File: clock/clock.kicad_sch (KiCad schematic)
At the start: 15 parts, among them Y1 Crystal_16MHz

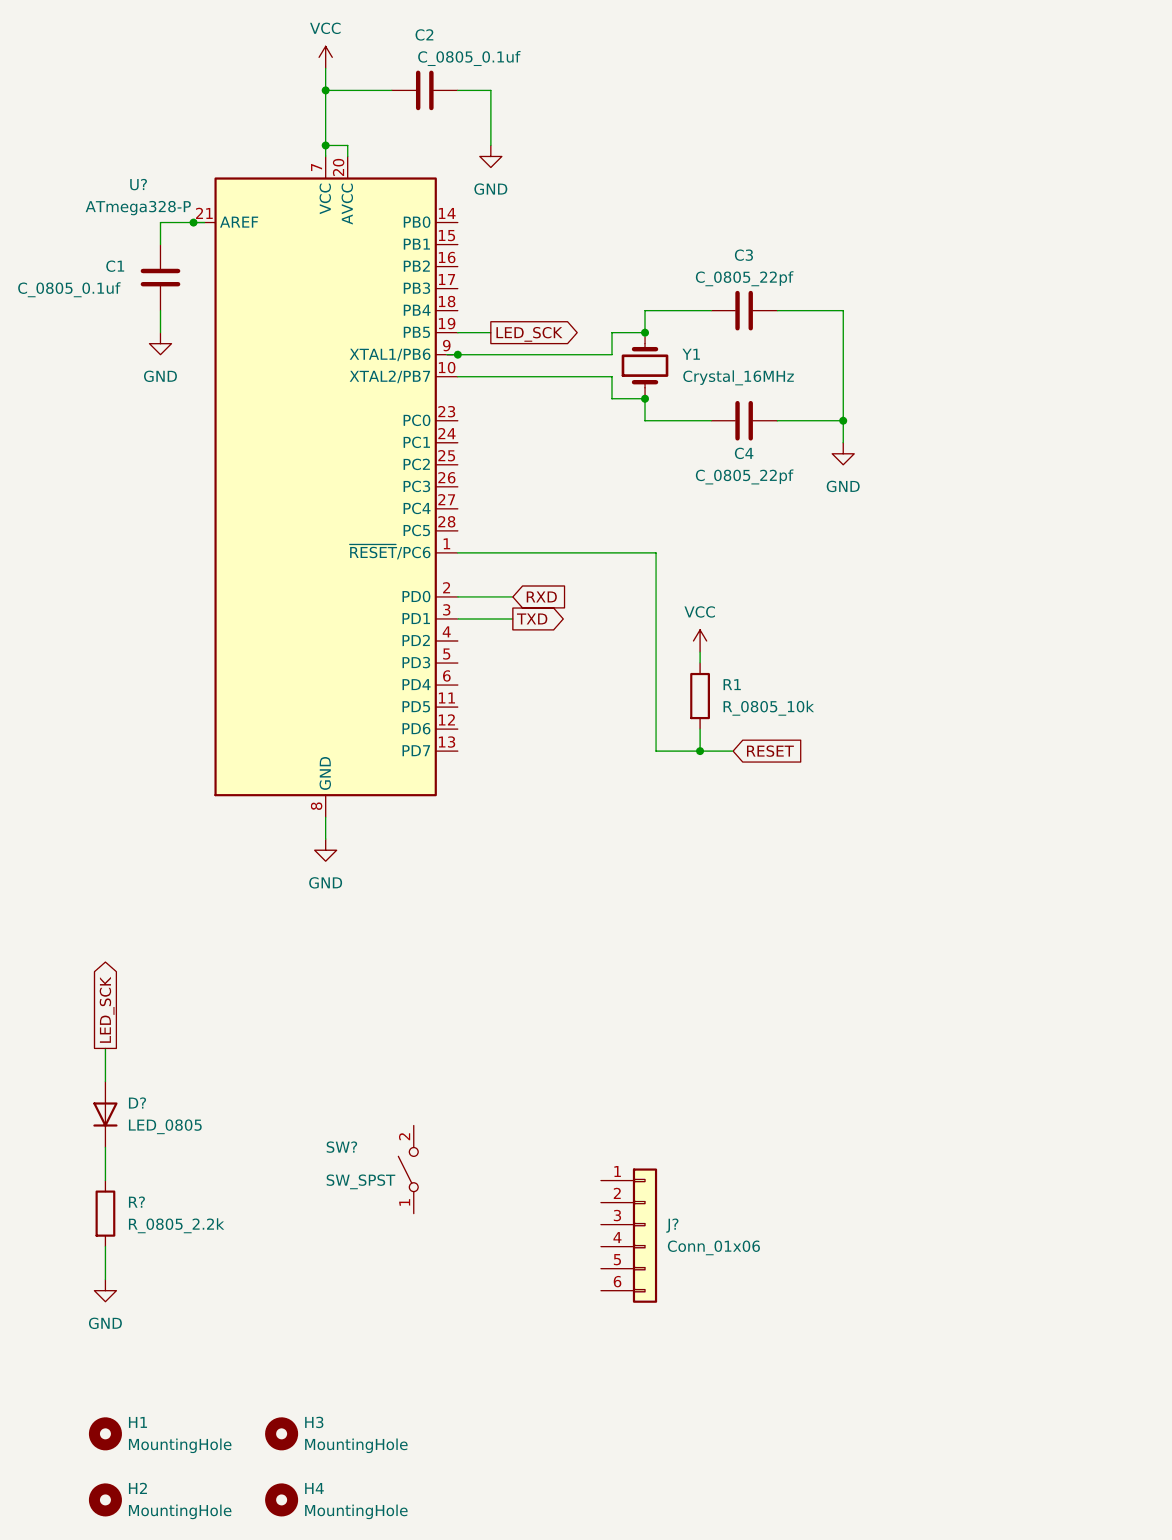
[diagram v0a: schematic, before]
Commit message: ch
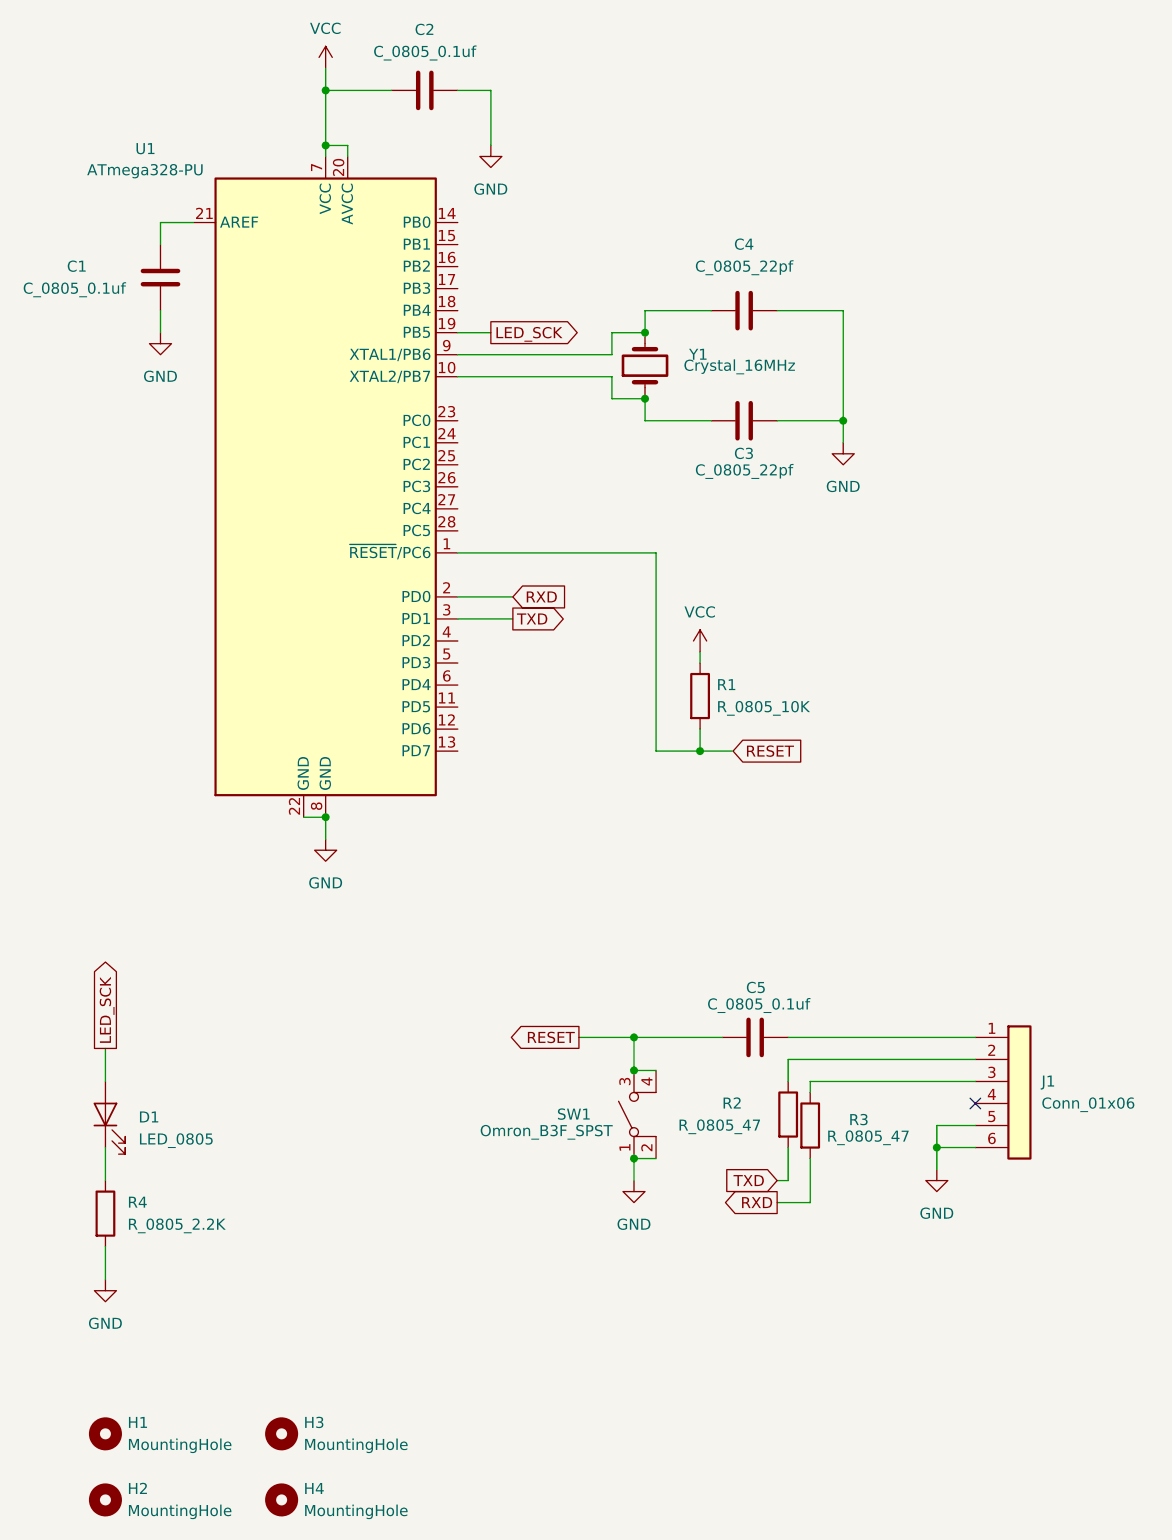
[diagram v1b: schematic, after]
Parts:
- removed C1, C2: C_0805_0.1uf, symbol Device:C
- removed C3, C4: C_0805_22pf, symbol Device:C
- removed D?: LED_0805, symbol Device:D
- removed J?: Conn_01x06, symbol Connector_Generic:Conn_01x06
- removed R1: R_0805_10k, symbol Device:R
- removed R?: R_0805_2.2k, symbol Device:R
- removed SW?: SW_SPST, symbol Switch:SW_SPST
- removed U?: ATmega328-P, Package_DIP:DIP-28_W7.62mm, symbol MCU_Microchip_ATmega:ATmega328-P
- removed Y1: Crystal_16MHz, symbol Device:Crystal
- added C1, C2, C5: C_0805_0.1uf, footprints:C_0805_2012Metric, symbol HPS:C_0805_0.1uf
- added C3, C4: C_0805_22pf, footprints:C_0805_2012Metric, symbol HPS:C_0805_22pf
- added D1: LED_0805, footprints:LED_0805_2012Metric, symbol HPS:LED_0805
- added J1: Conn_01x06, footprints:PinHeader_1x06_P2.54mm_Vertical, symbol HPS:Conn_01x06
- added R1: R_0805_10K, footprints:R_0805_2012Metric, symbol HPS:R_0805_10K
- added R2, R3: R_0805_47, footprints:R_0805_2012Metric, symbol HPS:R_0805_47
- added R4: R_0805_2.2K, footprints:R_0805_2012Metric, symbol HPS:R_0805_2.2K
- added SW1: Omron_B3F_SPST, footprints:SW_SPST_Omron_B3FS-100xP, symbol HPS:Omron_B3F_SPST
- added U1: ATmega328-PU, footprints:DIP-28_W7.62mm, symbol HPS:ATmega328-PU
- added Y1: Crystal_16MHz, footprints:Crystal_SMD_HC49-SD, symbol HPS:Crystal_16MHz
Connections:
- net GND: now also C1.2, C2.2, C3.2, C4.2, J1.5 (Pin_5), J1.6 (Pin_6), R4.2, SW1.1 (A), SW1.2 (A), U1.22 (GND), U1.8 (GND)
- net LED_SCK: now also D1.2 (A), U1.19 (PB5)
- net RESET: now also C5.1, R1.2, SW1.3 (B), SW1.4 (B), U1.1 (~{RESET}/PC6)
- net RXD: now also R3.2, U1.2 (PD0)
- net TXD: now also R2.2, U1.3 (PD1)
- net VCC: now also C2.1, R1.1, U1.20 (AVCC), U1.7 (VCC)
- new net: D1.1 (K), R4.1
- new net: J1.2 (Pin_2), R2.1
- new net: C3.1, U1.10 (XTAL2/PB7), Y1.1
- new net: C1.1, U1.21 (AREF)
- new net: C4.1, U1.9 (XTAL1/PB6), Y1.2
- new net: C5.2, J1.1 (Pin_1)
- new net: J1.3 (Pin_3), R3.1
- no-connect marks 0 -> 1
